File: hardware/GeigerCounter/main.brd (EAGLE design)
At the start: 53.8 x 32.8 mm, 34 parts, among them T4 

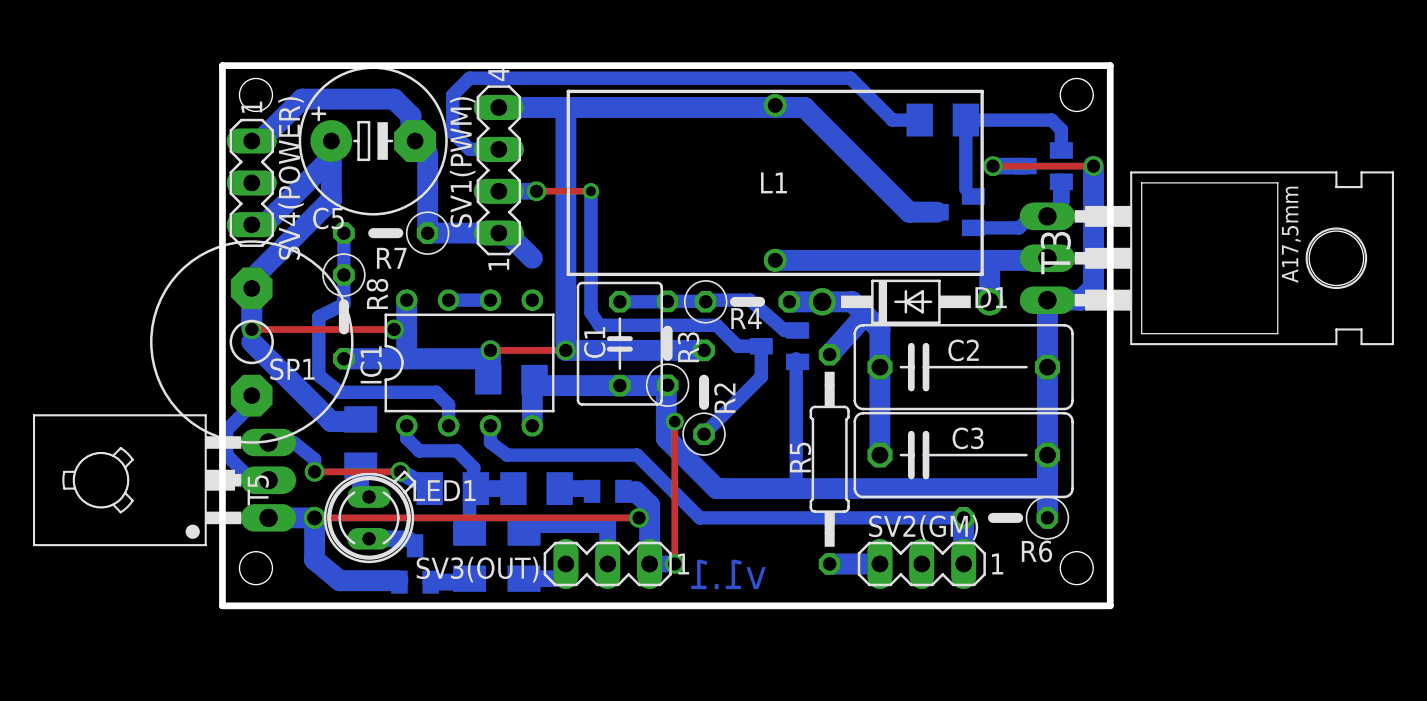
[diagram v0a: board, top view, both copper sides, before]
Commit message: Fixed PCB.
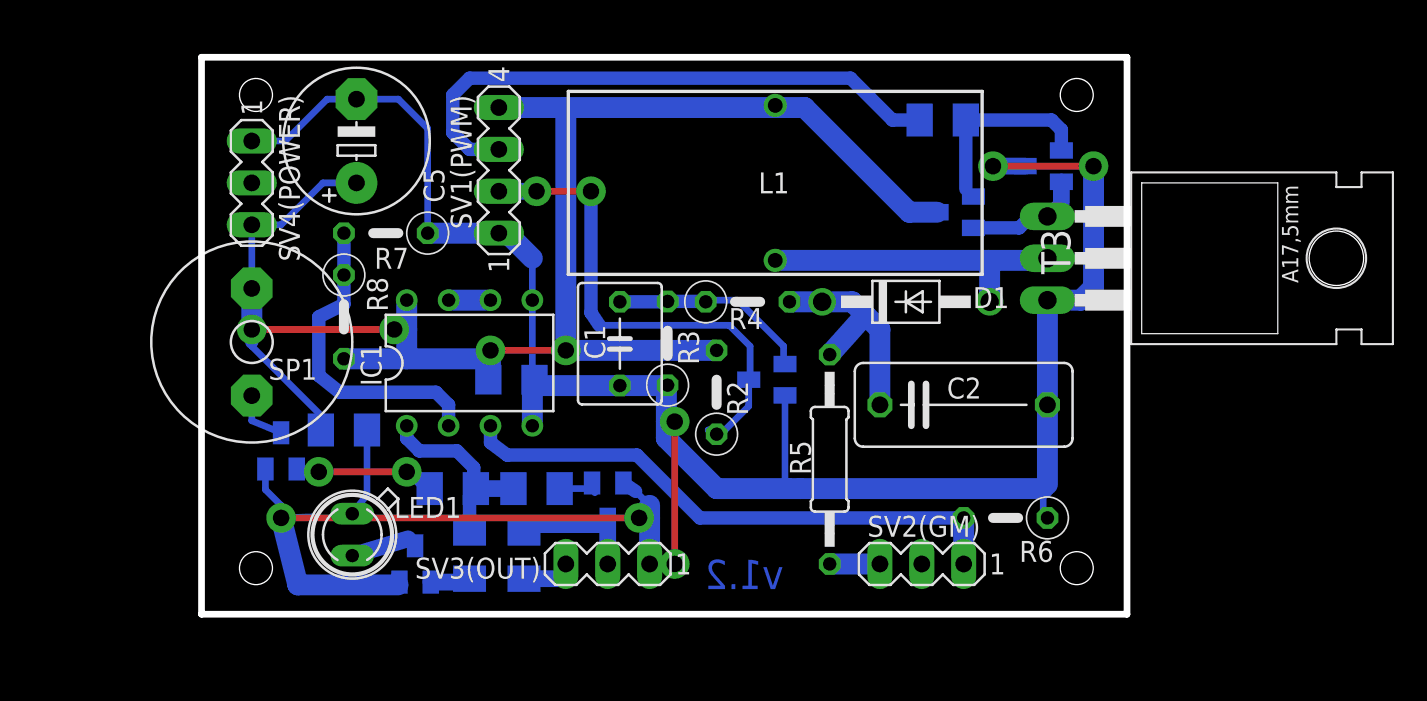
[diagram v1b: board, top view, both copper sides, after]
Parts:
- removed C3: (no value), resistor:C102-054X133
- T5: device transistor:TO126 -> transistor-npn:SOT23
- moved T5 6.11 mm to (44.2, 13.0), flipped to the bottom, turned to 0 degrees
- moved C2 2.29 mm to (85.6, 15.7)
- moved T4 2.17 mm to (73.7, 17.3)
- moved LED1 1.44 mm to (48.5, 7.87)
- moved R12 1.27 mm to (48.0, 14.2), turned to 0 degrees
- moved C5 1.02 mm to (48.8, 31.8), turned to 90 degrees
- moved R2 0.76 mm to (70.6, 16.5)
- moved T7 0.51 mm to (64.0, 9.91)
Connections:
- net N$12: no longer C3.1
- net N$13: now also T5.3; no longer T5.2
- net N$5: now also T5.2; no longer C3.2, T5.1
- net N$9: now also T5.1; no longer T5.3
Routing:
- net N$7: track 112.1 -> 104.4 mm
- net N$5: track 157.8 -> 164.8 mm
- net N$13: track 7.41 -> 3.45 mm
- net N$6: track 2.11 -> 5.39 mm
- net N$12: track 17.0 -> 14.0 mm
- net N$9: track 11.2 -> 8.56 mm
- net N$3: track 2.97 -> 4.13 mm
- net N$4: track 8.47 -> 9.40 mm
- net N$1: track 2.23 -> 3.10 mm
- net N$10: track 11.5 -> 12.2 mm
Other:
- board size 53.8 x 32.8 mm -> 56.1 x 33.8 mm
- board text added: "v1.2"
- board text removed: "v1.1"

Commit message: Built and tested version.
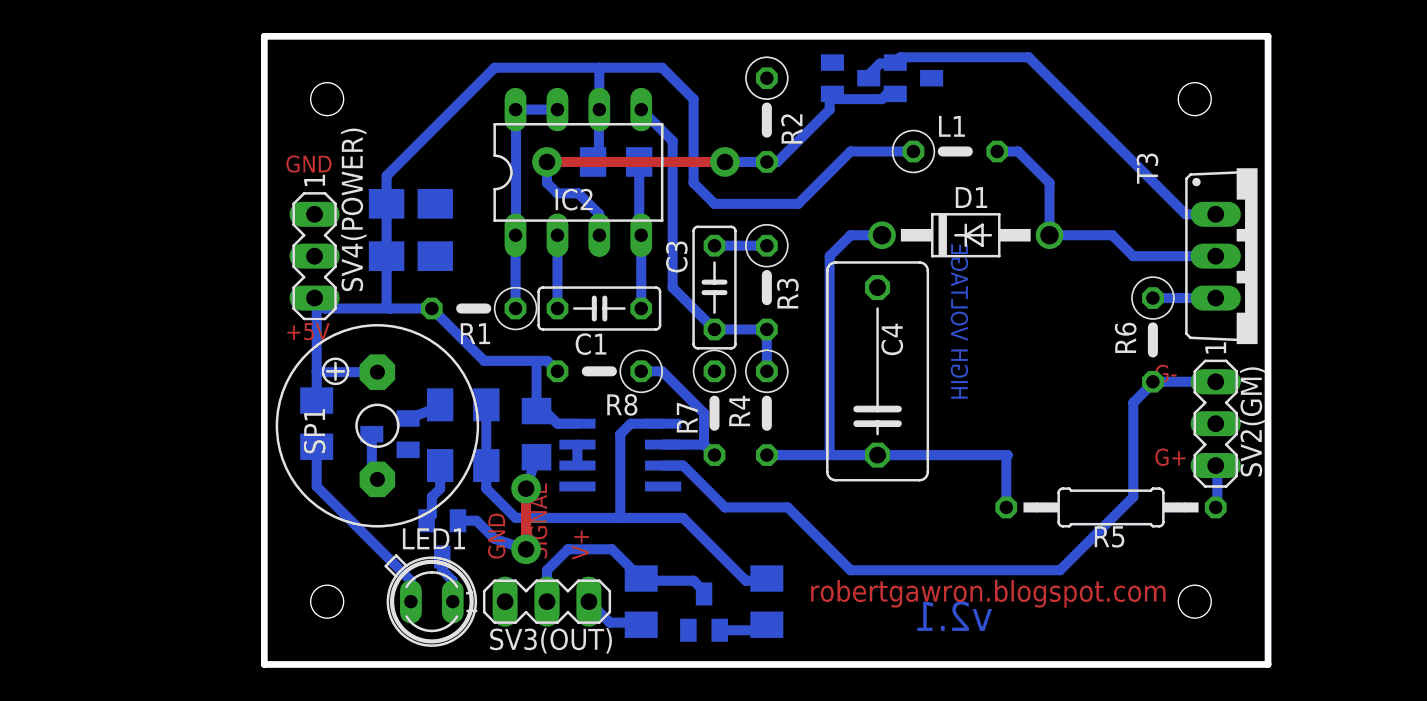
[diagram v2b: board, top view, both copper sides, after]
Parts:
- removed SV1(PWM): (no value), con-lstb:MA04-1
- removed T4, T5: (no value), transistor-npn:SOT23
- added C3: (no value), resistor:C050-025X075
- added C6, C7: 330u, resistor:A/3216-18W
- added D2: BAS40, diode:SOT23
- added IC2: (no value), ic-package:DIL08
- C1: device resistor:C050-050X075 -> resistor:C050-025X075
- C2: device resistor:C102-054X133 -> resistor:C3216
- C4: device resistor:C3216 -> resistor:C102-064X133
- C5: value (none) -> 100n; device resistor:E5-8,5 -> resistor:C3216
- IC1: value (none) -> LM358D; device linear:DIL08 -> linear:SO08
- L1: device resistor:TJ5-U1 -> resistor:0207/5V
- R1: device resistor:M1206 -> resistor:0207/5V
- R10, R11, R9: value (none) -> 1k
- R12: value (none) -> 510R
- SP1: value (none) -> 8R; device buzzer:AL60P -> buzzer:KSS1201
- T3: value (none) -> IRF840; device transistor-fet:TO220 -> transistor-power:TO220BV
- moved T2 36.8 mm to (50.8, 14.0)
- moved R1 30.7 mm to (55.9, 21.6), flipped to the top
- moved C2 25.7 mm to (64.5, 30.5), flipped to the bottom, turned to 180 degrees
- moved R7 22.7 mm to (70.5, 15.2), turned to 270 degrees
- moved C4 22.2 mm to (80.4, 17.8), flipped to the top, turned to 90 degrees
- moved C5 20.9 mm to (59.7, 14.0), flipped to the bottom, turned to 270 degrees
- moved SV2(GM) 19.8 mm to (100.9, 14.6), turned to 270 degrees
- moved R5 17.3 mm to (94.5, 9.53), turned to 0 degrees
- moved R2 16.8 mm to (73.7, 33.0), turned to 270 degrees
- moved R8 15.8 mm to (63.5, 17.8), turned to 180 degrees
- moved R9 15.6 mm to (73.7, 3.81), turned to 270 degrees
- moved R6 14.0 mm to (97.1, 19.7), turned to 270 degrees
- moved L1 11.1 mm to (85.1, 31.1), turned to 0 degrees
- moved IC1 10.7 mm to (64.8, 12.7), flipped to the bottom, turned to 270 degrees
- moved T1 9.51 mm to (82.5, 35.6), turned to 90 degrees
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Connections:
- removed net N$14: R1.1, SV1(PWM).3
- removed net N$7: C4.1, C5.+, IC1.8, L1.1, R12.2, R2.2, R8.2, SP1.1, SV1(PWM).4, SV4(POWER).3, T2.3
- new net V+: C2.1, C5.1, C6.+, C7.+, IC1.8, IC2.6, L1.1, R1.2, R12.2, R8.2, SP1.+, SV4(POWER).3
- new net V-: C1.2, C2.2, C3.2, C4.2, C5.2, C6.-, C7.-, IC1.4, IC1.5, IC2.4, R2.1, R3.1, R6.1, R7.1, SV3(OUT).1, SV4(POWER).1, T1.C, T2.2, T3.S, T6.2, T7.2
- net N$10: now also R11.2, T2.1; no longer C1.1, R3.2, R4.1, T4.1
- net N$11: now also IC2.1, IC2.7, IC2.8, R1.1; no longer R2.1, SV1(PWM).2, T4.3
- net N$12: now also C4.1; no longer C2.1
- net N$13: now also C3.1, IC2.5, R3.2, R4.1; no longer SP1.2, T5.3
- net N$15: now also T3.D; no longer T3.2
- net N$16: now also D2.3, T3.G; no longer T2.2, T3.1
- net N$18: now also D2.1, IC2.3, R2.2; no longer R1.2, T2.1
- net N$5: now also C1.1, IC2.2; no longer C1.2, C2.2, C4.2, C5.-, IC1.4, IC1.5, R3.1, R6.1, R7.1, SV1(PWM).1, SV3(OUT).1, SV4(POWER).1, T1.C, T3.3, T4.2, T5.2, T6.2, T7.2
- net N$9: now also SP1.-, T2.3; no longer R11.2, T5.1
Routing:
- net N$5: track 164.8 -> 4.45 mm, vias 6 -> 0
- net N$7: track 104.4 -> 0.00 mm, vias 4 -> 0
- net V+: track 0.00 -> 89.3 mm
- net N$14: track 35.3 -> 0.00 mm
- net V-: track 0.00 -> 26.3 mm, vias 0 -> 2
- net N$8: track 12.0 -> 34.1 mm
- net N$12: track 14.0 -> 33.6 mm
- net N$16: track 7.22 -> 25.7 mm
- net N$18: track 12.2 -> 30.1 mm, vias 0 -> 2
- net N$13: track 3.45 -> 20.9 mm
- net N$11: track 30.8 -> 14.6 mm, vias 2 -> 0
- net N$10: track 12.2 -> 2.14 mm
- net N$17: track 34.3 -> 44.3 mm
- net N$19: track 19.4 -> 10.1 mm
- net N$6: track 5.39 -> 11.8 mm
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- added copper zone on layer 16, net V-
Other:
- board size 56.1 x 33.8 mm -> 60.9 x 38.1 mm
- board text added: "+5V"
- board text added: "G+"
- board text added: "G-"
- board text added: "GND"
- board text added: "HIGH VOLTAGE"
- board text added: "SIGNAL"
- board text added: "V+"
- board text added: "robertgawron.blogspot.com"
- board text added: "v2.1"
- board text removed: "v1.2"
